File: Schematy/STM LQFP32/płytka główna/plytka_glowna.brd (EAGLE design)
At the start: 150.5 x 72.4 mm, 53 parts, among them IC1 LM1117-3.3V, IC2 74HC595D

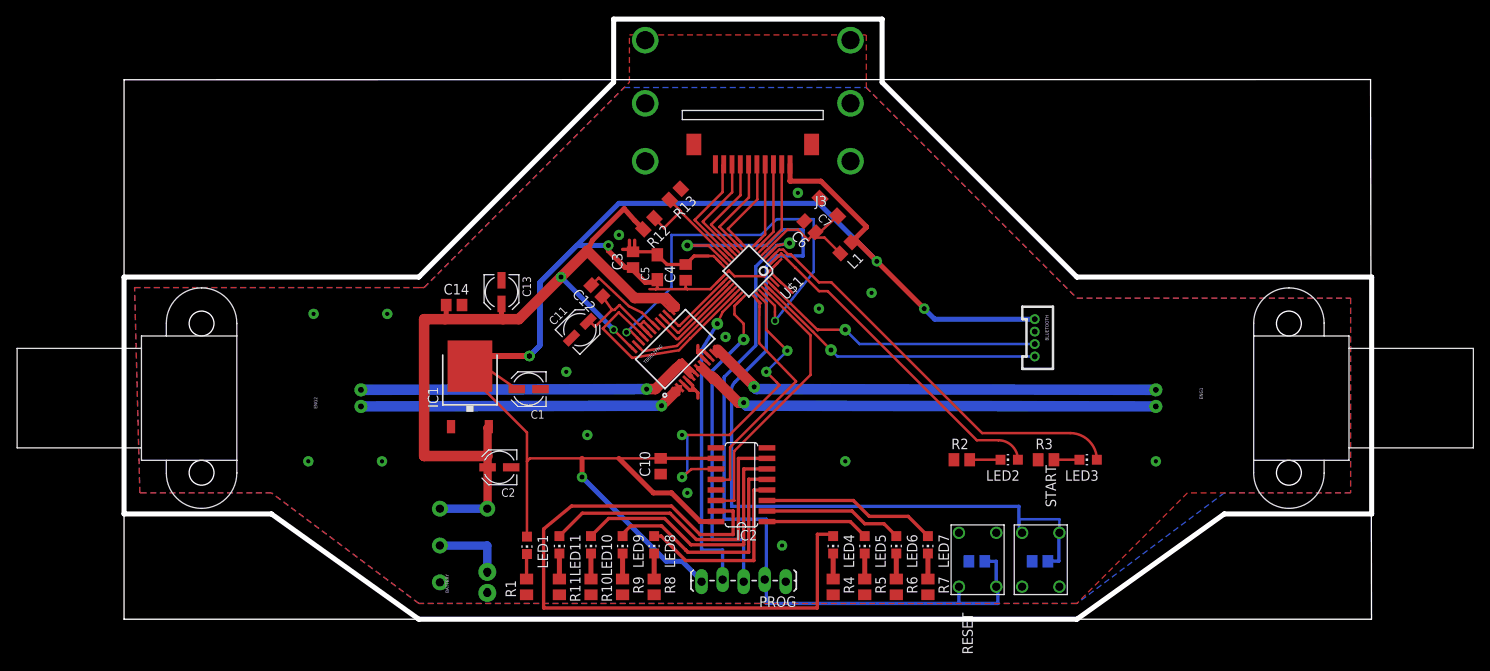
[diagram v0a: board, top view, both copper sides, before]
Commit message: poprawiona płytka główna
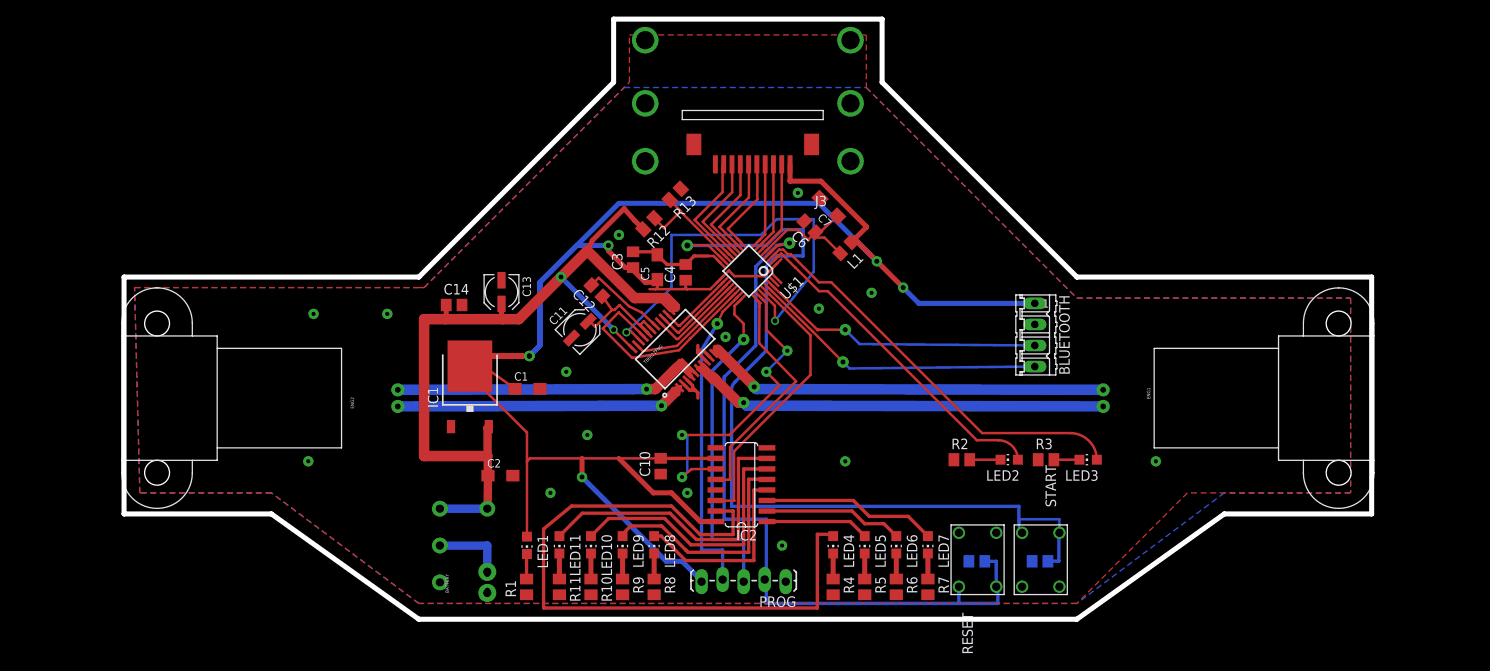
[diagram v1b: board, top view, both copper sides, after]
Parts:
- BLUETOOTH: device SparkFun-Connectors:1X04-1.5MM_JST -> con-amp-quick:04P
- C1, C2: device rcl:UD-4X5,8_NICHICON -> rcl:SMC_A
- moved ENG1 6.35 mm to (118.1, 26.7)
- moved ENG2 4.45 mm to (33.0, 26.7)
- moved BLUETOOTH 1.91 mm to (109.9, 34.3)
- moved C2 1.01 mm to (45.4, 17.3), turned to 0 degrees
- moved U$4 0.64 mm to (6.99, 26.7), turned to 270 degrees
- moved C1 0.15 mm to (48.7, 27.8), turned to 0 degrees
- turned U$3 to 90 degrees
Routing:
- net N$7: track 59.6 -> 53.2 mm
- net N$9: track 55.5 -> 49.2 mm
- net N$11: track 39.6 -> 35.2 mm
- net N$6: track 44.4 -> 40.0 mm
- net VSS: track 14.5 -> 12.0 mm
- net N$22: track 1.27 -> 0.00 mm
- net N$21: track 1.27 -> 0.00 mm
- net +3V3: track 196.3 -> 195.3 mm
- net N$23: track 0.88 -> 0.00 mm
- net BLUETOOTH_TX: track 35.5 -> 36.1 mm
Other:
- outline, holes or cut-outs redrawn
